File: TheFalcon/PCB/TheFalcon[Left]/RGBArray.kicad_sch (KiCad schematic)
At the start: 63 parts, among them IC1 IS31FL3729-QFLS4-TR, J4 Conn_01x01

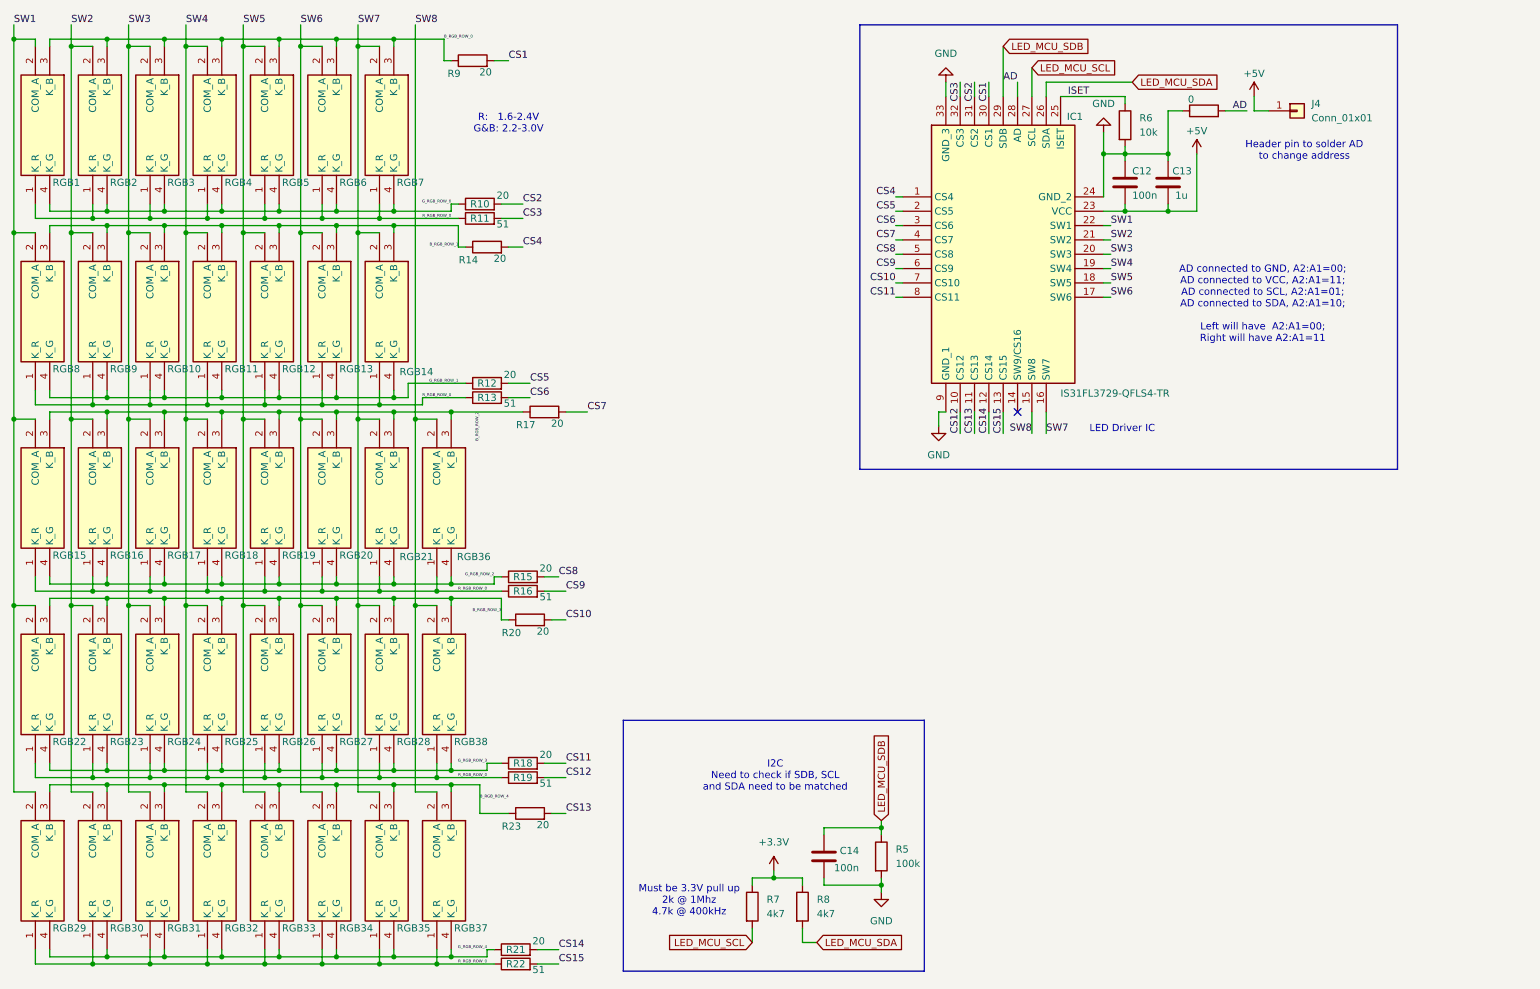
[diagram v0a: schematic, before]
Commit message: save
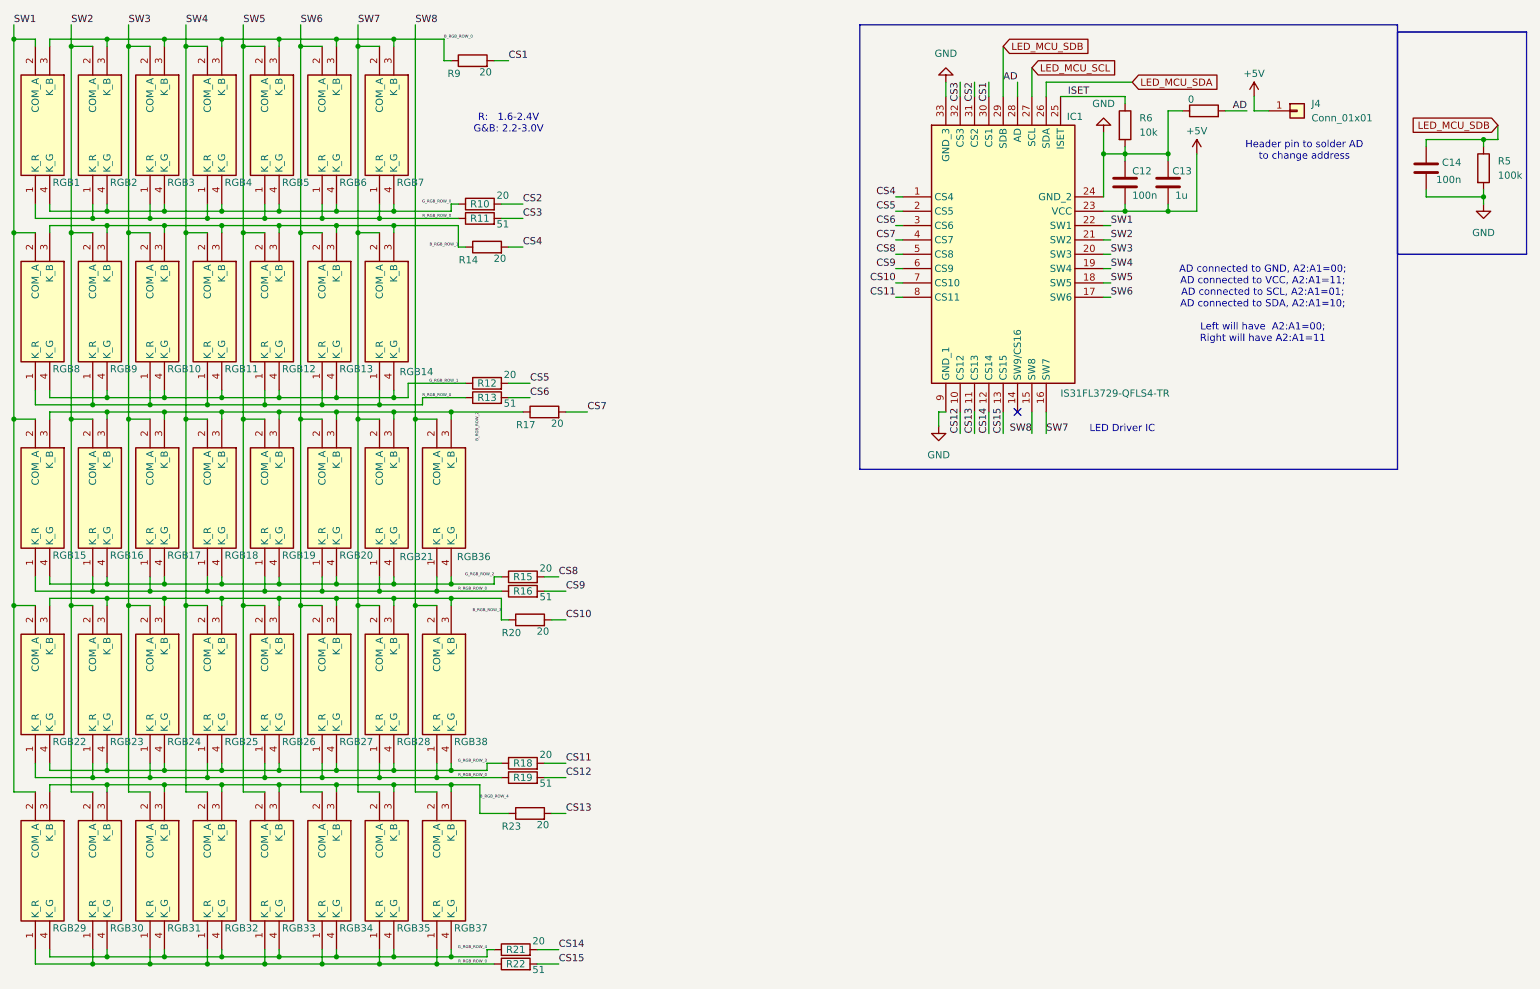
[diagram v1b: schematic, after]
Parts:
- removed R7, R8: 4k7, Resistor_SMD:R_0201_0603Metric, symbol Device:R
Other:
- note removed: "I2C Need to check if SDB, SCL and SDA need to be matched"
- note removed: "Must be 3.3V pull up 2k @ 1Mhz 4.7k @ 400kHz"
- moved on the sheet: C14, R5
